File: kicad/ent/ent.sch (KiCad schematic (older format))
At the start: 28 parts, among them J1 Conn_01x04_Male, J2 Conn_01x03_Male, J3 Conn_01x03_Male, J4 Conn_01x12_Male, J5 Conn_01x04_Male, J6 Conn_01x03_Male, J7 Conn_01x03_Male, SW1 SW_SPDT, SW2 SW_Push, U1 TPS62172DSG, U2 LIS2DHTR, U3 STM32F030K6Tx

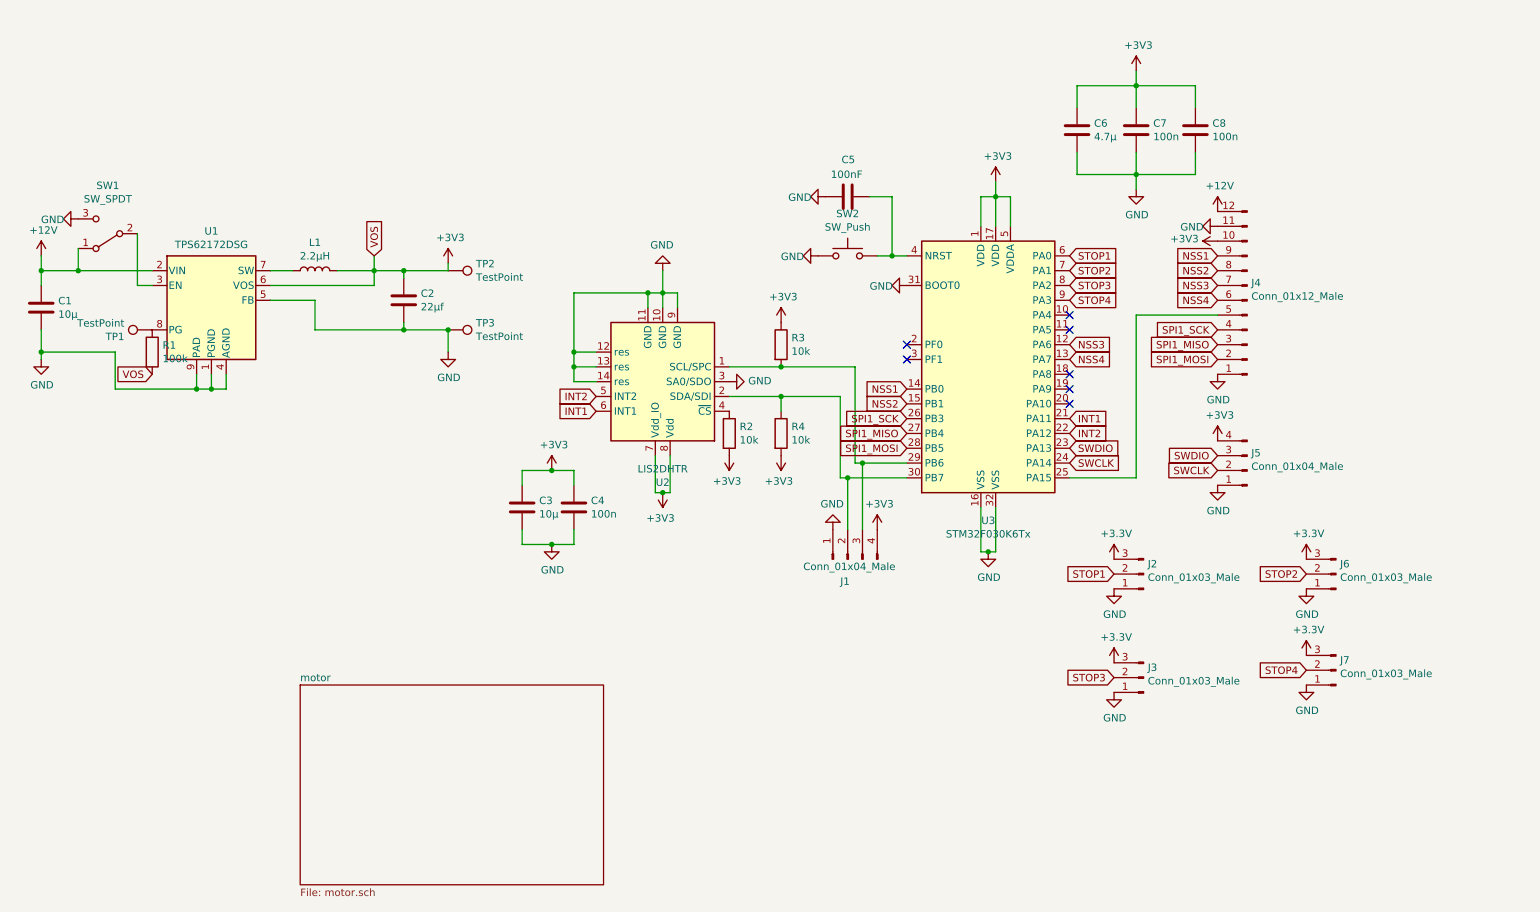
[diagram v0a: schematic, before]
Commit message: soft update + pcb main try 1
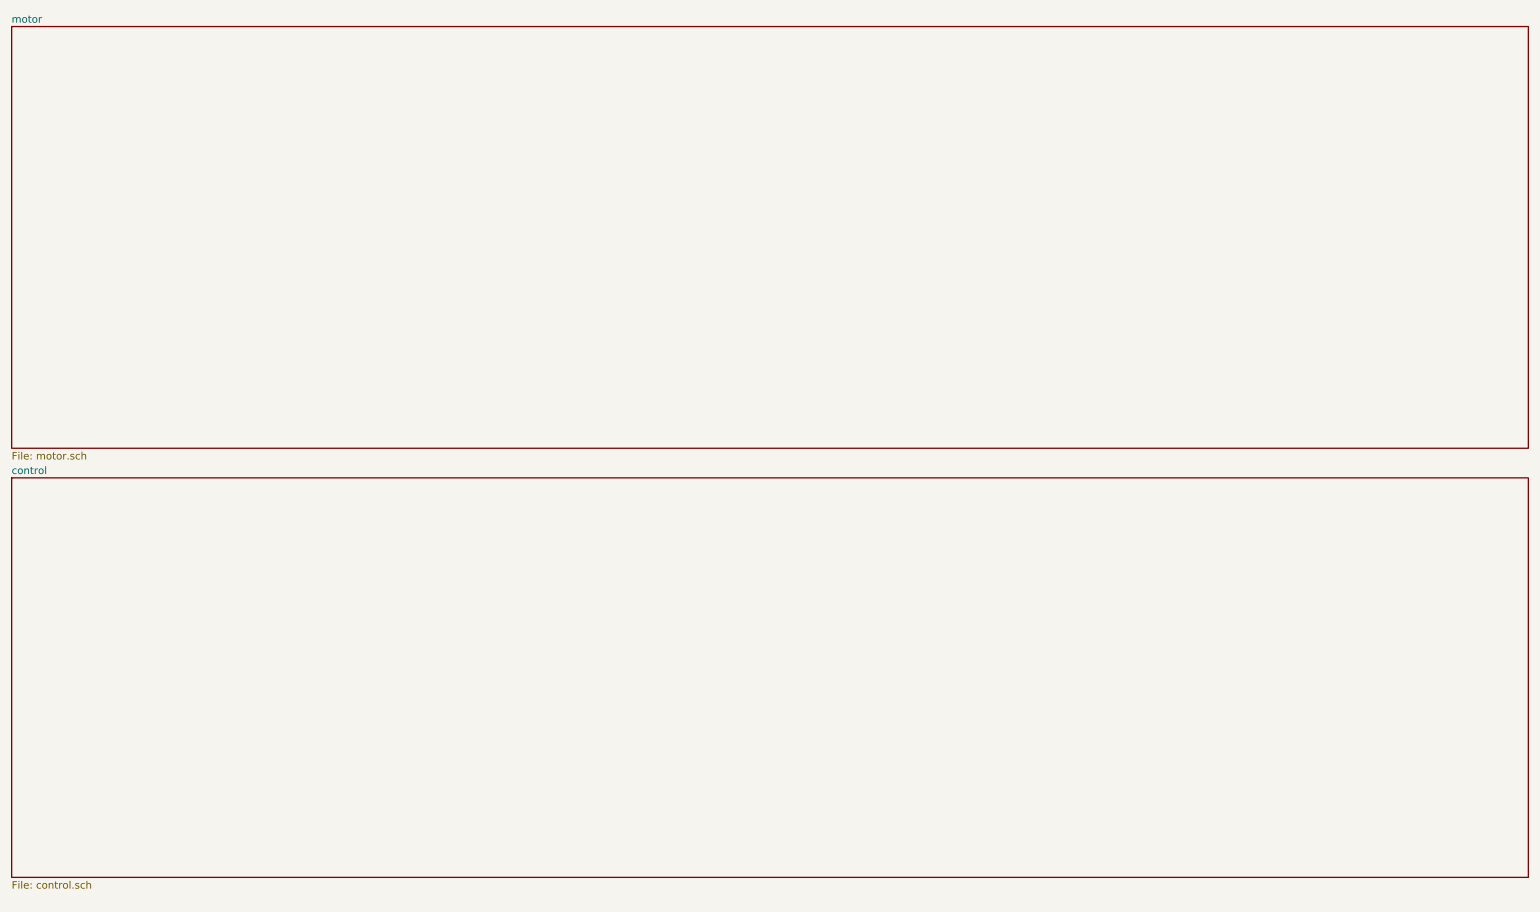
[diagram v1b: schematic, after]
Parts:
- removed C1, C3: 10µ, Capacitor_SMD:C_0805_2012Metric_Pad1.15x1.40mm_HandSolder, symbol Device:C
- removed C2: 22µf, Capacitor_SMD:C_0805_2012Metric_Pad1.15x1.40mm_HandSolder, symbol Device:C
- removed C4, C7, C8: 100n, Capacitor_SMD:C_0805_2012Metric_Pad1.15x1.40mm_HandSolder, symbol Device:C
- removed C5: 100nF, Capacitor_SMD:C_0805_2012Metric_Pad1.15x1.40mm_HandSolder, symbol Device:C
- removed C6: 4.7µ, Capacitor_SMD:C_0805_2012Metric_Pad1.15x1.40mm_HandSolder, symbol Device:C
- removed J1, J5: Conn_01x04_Male, Connector_JST:JST_XH_B4B-XH-A_1x04_P2.50mm_Vertical, symbol Connector:Conn_01x04_Male
- removed J2, J3, J6, J7: Conn_01x03_Male, Connector_JST:JST_XH_B3B-XH-A_1x03_P2.50mm_Vertical, symbol Connector:Conn_01x03_Male
- removed J4: Conn_01x12_Male, Connector_JST:JST_XH_B12B-XH-A_1x12_P2.50mm_Vertical, symbol Connector:Conn_01x12_Male
- removed L1: 2.2µH, Inductor_SMD:L_0805_2012Metric_Pad1.15x1.40mm_HandSolder, symbol Device:L
- removed R1: 100k, Resistor_SMD:R_0805_2012Metric_Pad1.15x1.40mm_HandSolder, symbol Device:R
- removed R2, R3, R4: 10k, Resistor_SMD:R_0805_2012Metric_Pad1.15x1.40mm_HandSolder, symbol Device:R
- removed SW1: SW_SPDT, Connector_PinHeader_2.54mm:PinHeader_1x03_P2.54mm_Vertical, symbol Switch:SW_SPDT
- removed SW2: SW_Push, Button_Switch_SMD:SW_SPST_PTS645, symbol Switch:SW_Push
- removed TP1, TP2, TP3: TestPoint, TestPoint:TestPoint_Pad_D2.0mm, symbol Connector:TestPoint
- removed U1: TPS62172DSG, Package_SON:WSON-8-1EP_2x2mm_P0.5mm_EP0.9x1.6mm_ThermalVias, symbol Regulator_Switching:TPS62172DSG
- removed U2: LIS2DHTR, Package_LGA:LGA-14_2x2mm_P0.35mm_LayoutBorder3x4y, symbol ent-rescue:LIS2DHTR-ian
- removed U3: STM32F030K6Tx, Package_QFP:LQFP-32_7x7mm_P0.8mm, symbol MCU_ST_STM32F0:STM32F030K6Tx
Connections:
- no-connect marks 7 -> 0
